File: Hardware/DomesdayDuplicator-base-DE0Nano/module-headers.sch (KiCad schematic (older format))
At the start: 20 parts, among them J401 MOD0 Back, J402 MOD0 Back, J403 MOD0 Front, J404 MOD1 Front

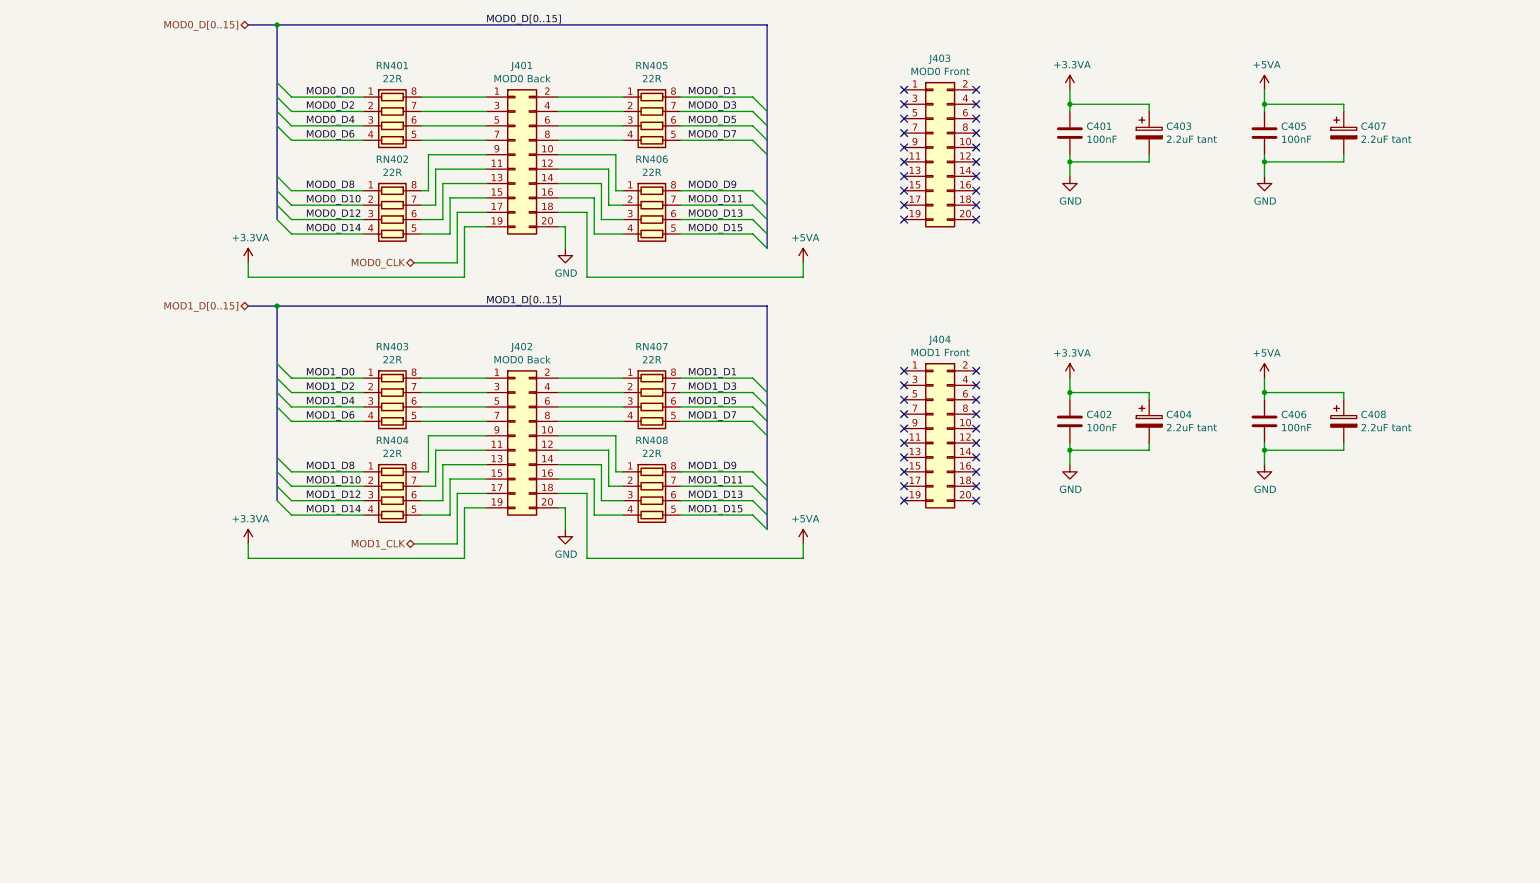
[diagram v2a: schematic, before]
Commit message: Mechanical set up of base board and basic routing
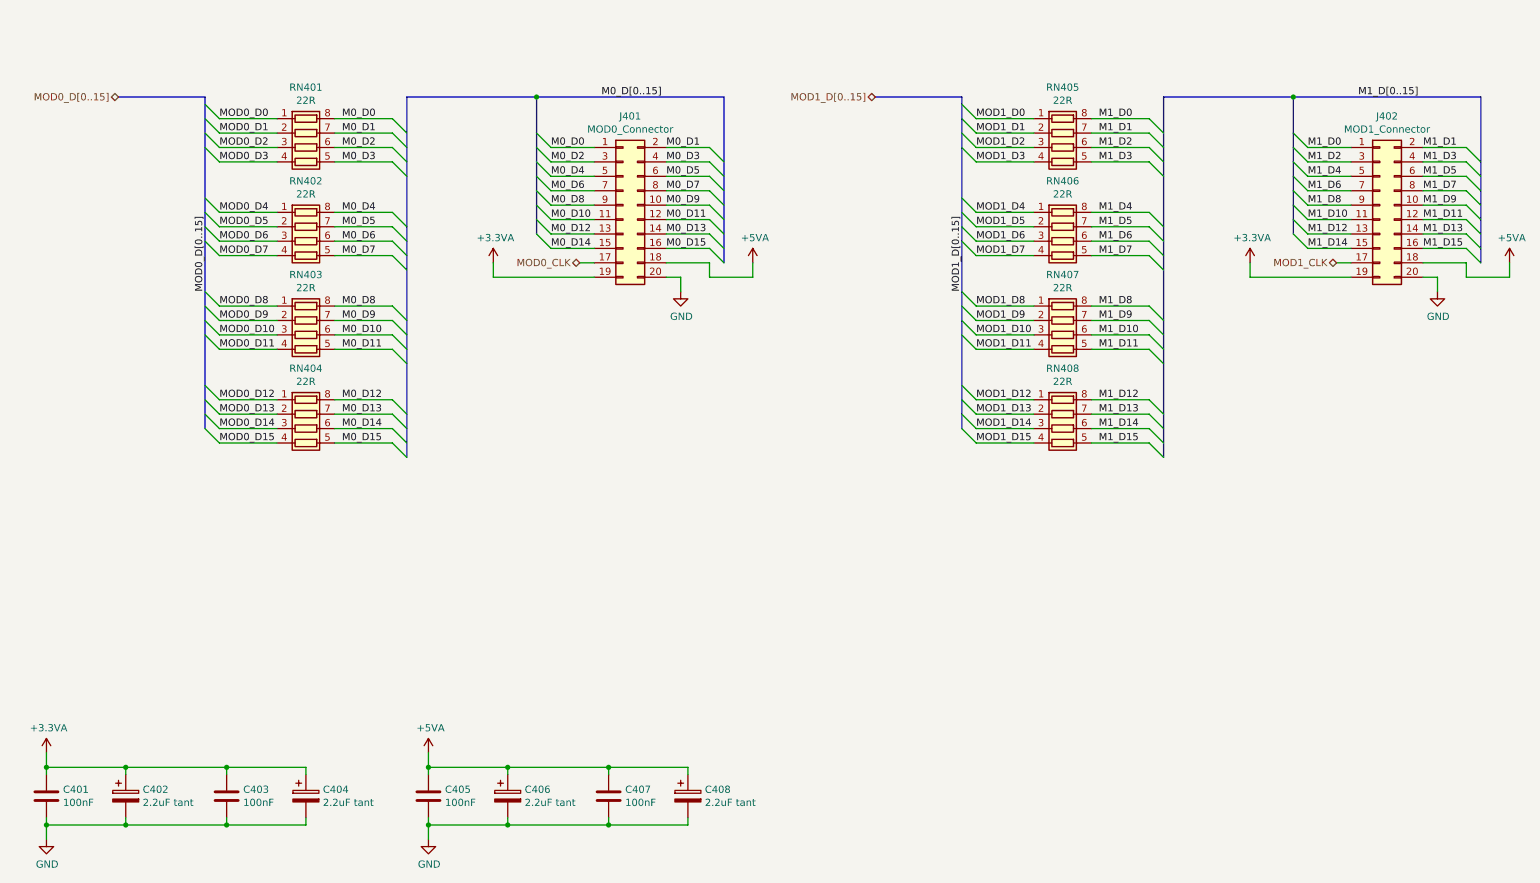
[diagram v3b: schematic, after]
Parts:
- removed C406: 100nF, Capacitor_SMD:C_0805_2012Metric, symbol Device:C
- removed C407: 2.2uF tant, Capacitor_Tantalum_SMD:CP_EIA-3216-18_Kemet-A, symbol Device:CP
- removed J403: MOD0 Front, Connector_Hirose:Hirose_DF12_DF12C3.0-20DS-0.5V_2x10_P0.50mm_Vertical, symbol Connector_Generic:Conn_02x10_Odd_Even
- removed J404: MOD1 Front, Connector_Hirose:Hirose_DF12_DF12C3.0-20DS-0.5V_2x10_P0.50mm_Vertical, symbol Connector_Generic:Conn_02x10_Odd_Even
- removed RN403, RN404: 22R, Resistor_SMD:R_Array_Convex_4x1206, symbol Device:R_Pack04
- added C406: 2.2uF tant, Capacitor_Tantalum_SMD:CP_EIA-3216-18_Kemet-A, symbol Device:CP
- added C407: 100nF, Capacitor_SMD:C_0805_2012Metric, symbol Device:C
- added RN405, RN406: 22R, Resistor_SMD:R_Array_Convex_4x1206, symbol Device:R_Pack04
- J401: value MOD0 Back -> MOD0_Connector; footprint Connector_Hirose:Hirose_DF12_DF12C3.0-20DS-0.5V_2x10_P0.50mm_Vertical -> Connector_IDC:IDC-Header_2x10_P2.54mm_Vertical
- J402: value MOD0 Back -> MOD1_Connector; footprint Connector_Hirose:Hirose_DF12_DF12C3.0-20DS-0.5V_2x10_P0.50mm_Vertical -> Connector_IDC:IDC-Header_2x10_P2.54mm_Vertical
- renumbered C403 to C402, C402 to C403, RN405 to RN403, RN406 to RN404
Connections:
- net +5VA: now also C406.1, C407.1
- net GND: now also C406.2, C407.2
- net MOD0_D1: now also RN401.2 (R2.1); no longer RN403.8 (R1.2)
- net MOD0_D10: now also RN403.3 (R3.1); no longer RN402.2 (R2.1)
- net MOD0_D11: now also RN403.4 (R4.1); no longer RN404.7 (R2.2)
- net MOD0_D12: now also RN404.1 (R1.1); no longer RN402.3 (R3.1)
- net MOD0_D13: now also RN404.2 (R2.1); no longer RN404.6 (R3.2)
- net MOD0_D14: now also RN404.3 (R3.1); no longer RN402.4 (R4.1)
- net MOD0_D15: now also RN404.4 (R4.1); no longer RN404.5 (R4.2)
- net MOD0_D2: now also RN401.3 (R3.1); no longer RN401.2 (R2.1)
- net MOD0_D3: now also RN401.4 (R4.1); no longer RN403.7 (R2.2)
- net MOD0_D4: now also RN402.1 (R1.1); no longer RN401.3 (R3.1)
- net MOD0_D5: now also RN402.2 (R2.1); no longer RN403.6 (R3.2)
- net MOD0_D6: now also RN402.3 (R3.1); no longer RN401.4 (R4.1)
- net MOD0_D7: now also RN402.4 (R4.1); no longer RN403.5 (R4.2)
- net MOD0_D8: now also RN403.1 (R1.1); no longer RN402.1 (R1.1)
- net MOD0_D9: now also RN403.2 (R2.1); no longer RN404.8 (R1.2)
- net MOD1_D0: now also RN405.1 (R1.1)
- net MOD1_D1: now also RN405.2 (R2.1); no longer RN407.8 (R1.2)
- net MOD1_D10: now also RN407.3 (R3.1)
- net MOD1_D11: now also RN407.4 (R4.1); no longer RN408.7 (R2.2)
- net MOD1_D12: now also RN408.1 (R1.1)
- net MOD1_D13: now also RN408.2 (R2.1); no longer RN408.6 (R3.2)
- net MOD1_D14: now also RN408.3 (R3.1)
- net MOD1_D15: now also RN408.4 (R4.1); no longer RN408.5 (R4.2)
- net MOD1_D2: now also RN405.3 (R3.1)
- net MOD1_D3: now also RN405.4 (R4.1); no longer RN407.7 (R2.2)
- net MOD1_D4: now also RN406.1 (R1.1)
- net MOD1_D5: now also RN406.2 (R2.1); no longer RN407.6 (R3.2)
- net MOD1_D6: now also RN406.3 (R3.1)
- net MOD1_D7: now also RN406.4 (R4.1); no longer RN407.5 (R4.2)
- net MOD1_D8: now also RN407.1 (R1.1)
- net MOD1_D9: now also RN407.2 (R2.1); no longer RN408.8 (R1.2)
- net M0_D3: now reaches RN401.5 (R4.2)
- net M0_D3: now also J401.4 (Pin_4); no longer J401.7 (Pin_7)
- net M0_D2: now reaches RN401.6 (R3.2)
- net M0_D2: now also J401.3 (Pin_3); no longer J401.5 (Pin_5)
- net M0_D1: now reaches RN401.7 (R2.2)
- net M0_D1: now also J401.2 (Pin_2); no longer J401.3 (Pin_3)
- net M0_D0: now reaches J401.1 (Pin_1), RN401.8 (R1.2)
- net M0_D14: now reaches J401.15 (Pin_15)
- net M0_D14: now also RN404.6 (R3.2); no longer RN402.5 (R4.2)
- net M0_D12: now reaches J401.13 (Pin_13)
- net M0_D12: now also RN404.8 (R1.2); no longer RN402.6 (R3.2)
- net M0_D10: now reaches J401.11 (Pin_11)
- net M0_D10: now also RN403.6 (R3.2); no longer RN402.7 (R2.2)
- net M0_D4: now reaches RN402.8 (R1.2)
- net M0_D4: now also J401.5 (Pin_5); no longer J401.9 (Pin_9)
- net M0_D5: now reaches J401.6 (Pin_6)
- net M0_D5: now also RN402.7 (R2.2); no longer RN403.3 (R3.1)
- net M0_D7: now reaches J401.8 (Pin_8)
- net M0_D7: now also RN402.5 (R4.2); no longer RN403.4 (R4.1)
- net M0_D9: now reaches J401.10 (Pin_10)
- net M0_D9: now also RN403.7 (R2.2); no longer RN404.1 (R1.1)
- net M0_D11: now reaches J401.12 (Pin_12)
- net M0_D11: now also RN403.5 (R4.2); no longer RN404.2 (R2.1)
- net M0_D13: now reaches J401.14 (Pin_14)
- net M0_D13: now also RN404.7 (R2.2); no longer RN404.3 (R3.1)
- net M0_D15: now reaches J401.16 (Pin_16)
- net M0_D15: now also RN404.5 (R4.2); no longer RN404.4 (R4.1)
- net M1_D0: now reaches J402.1 (Pin_1)
- net M1_D0: now also RN405.8 (R1.2)
- net M1_D9: now reaches J402.10 (Pin_10)
- net M1_D9: now also RN407.7 (R2.2); no longer RN408.1 (R1.1)
- net M1_D10: now reaches J402.11 (Pin_11)
- net M1_D10: now also RN407.6 (R3.2)
- net M1_D11: now reaches J402.12 (Pin_12)
- net M1_D11: now also RN407.5 (R4.2); no longer RN408.2 (R2.1)
- net M1_D12: now reaches J402.13 (Pin_13)
- net M1_D12: now also RN408.8 (R1.2)
- net M1_D13: now reaches J402.14 (Pin_14)
- net M1_D13: now also RN408.7 (R2.2); no longer RN408.3 (R3.1)
- net M1_D14: now reaches J402.15 (Pin_15)
- net M1_D14: now also RN408.6 (R3.2)
- net M1_D15: now reaches J402.16 (Pin_16)
- net M1_D15: now also RN408.5 (R4.2); no longer RN408.4 (R4.1)
- net M1_D1: now reaches J402.2 (Pin_2)
- net M1_D1: now also RN405.7 (R2.2); no longer RN407.1 (R1.1)
- net M1_D2: now reaches J402.3 (Pin_3)
- net M1_D2: now also RN405.6 (R3.2)
- net M1_D3: now reaches J402.4 (Pin_4)
- net M1_D3: now also RN405.5 (R4.2); no longer RN407.2 (R2.1)
- net M1_D4: now reaches J402.5 (Pin_5)
- net M1_D4: now also RN406.8 (R1.2)
- net M1_D5: now reaches J402.6 (Pin_6)
- net M1_D5: now also RN406.7 (R2.2); no longer RN407.3 (R3.1)
- net M1_D6: now reaches J402.7 (Pin_7)
- net M1_D6: now also RN406.6 (R3.2)
- net M1_D7: now reaches J402.8 (Pin_8)
- net M1_D7: now also RN406.5 (R4.2); no longer RN407.4 (R4.1)
- net M1_D8: now reaches J402.9 (Pin_9)
- net M1_D8: now also RN407.8 (R1.2)
- new net M0_D6: J401.7 (Pin_7), RN402.6 (R3.2)
- new net M0_D8: J401.9 (Pin_9), RN403.8 (R1.2)
- no-connect marks 40 -> 0
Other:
- moved on the sheet: C401, C402, C403, C404, J401, RN401, RN402, RN403, RN404
